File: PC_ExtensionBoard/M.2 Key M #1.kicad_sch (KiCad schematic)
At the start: 14 parts, among them J5 Bus_M.2_MDT180M03001

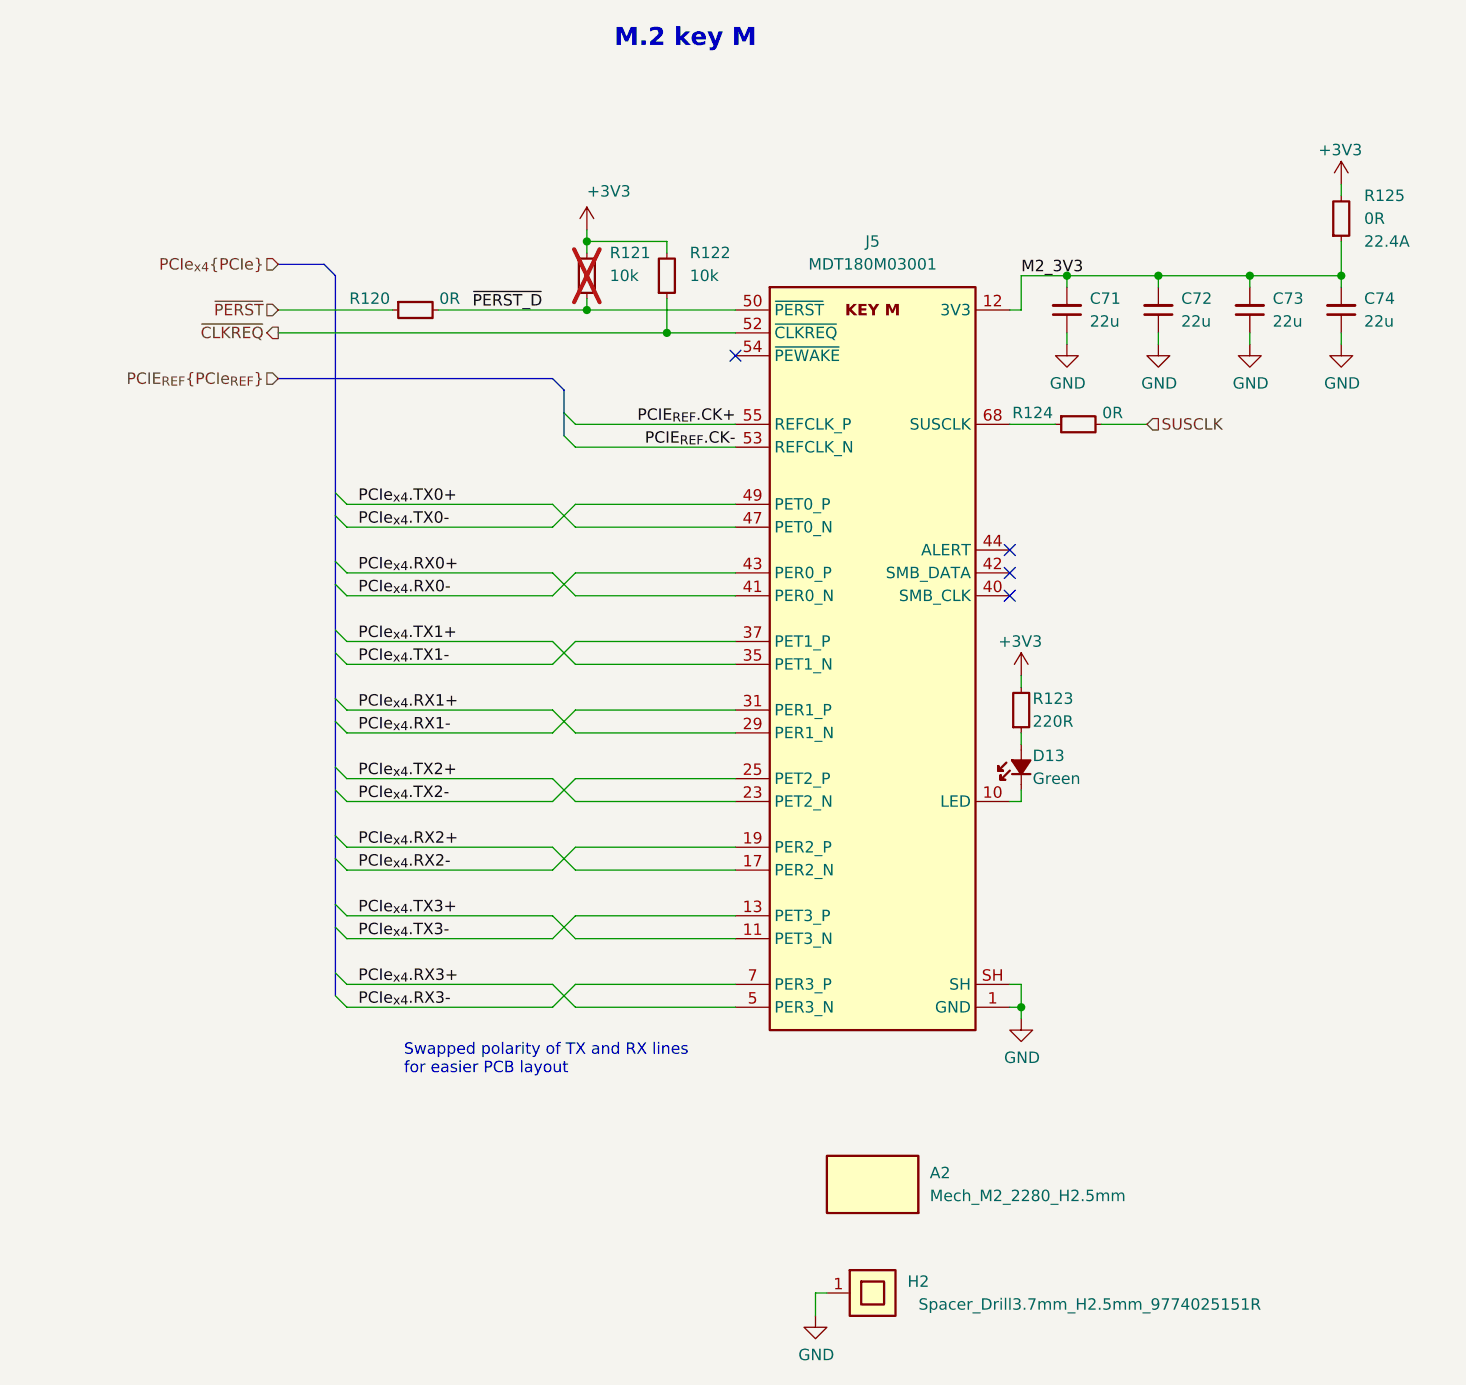
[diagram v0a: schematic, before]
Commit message: components placement R1
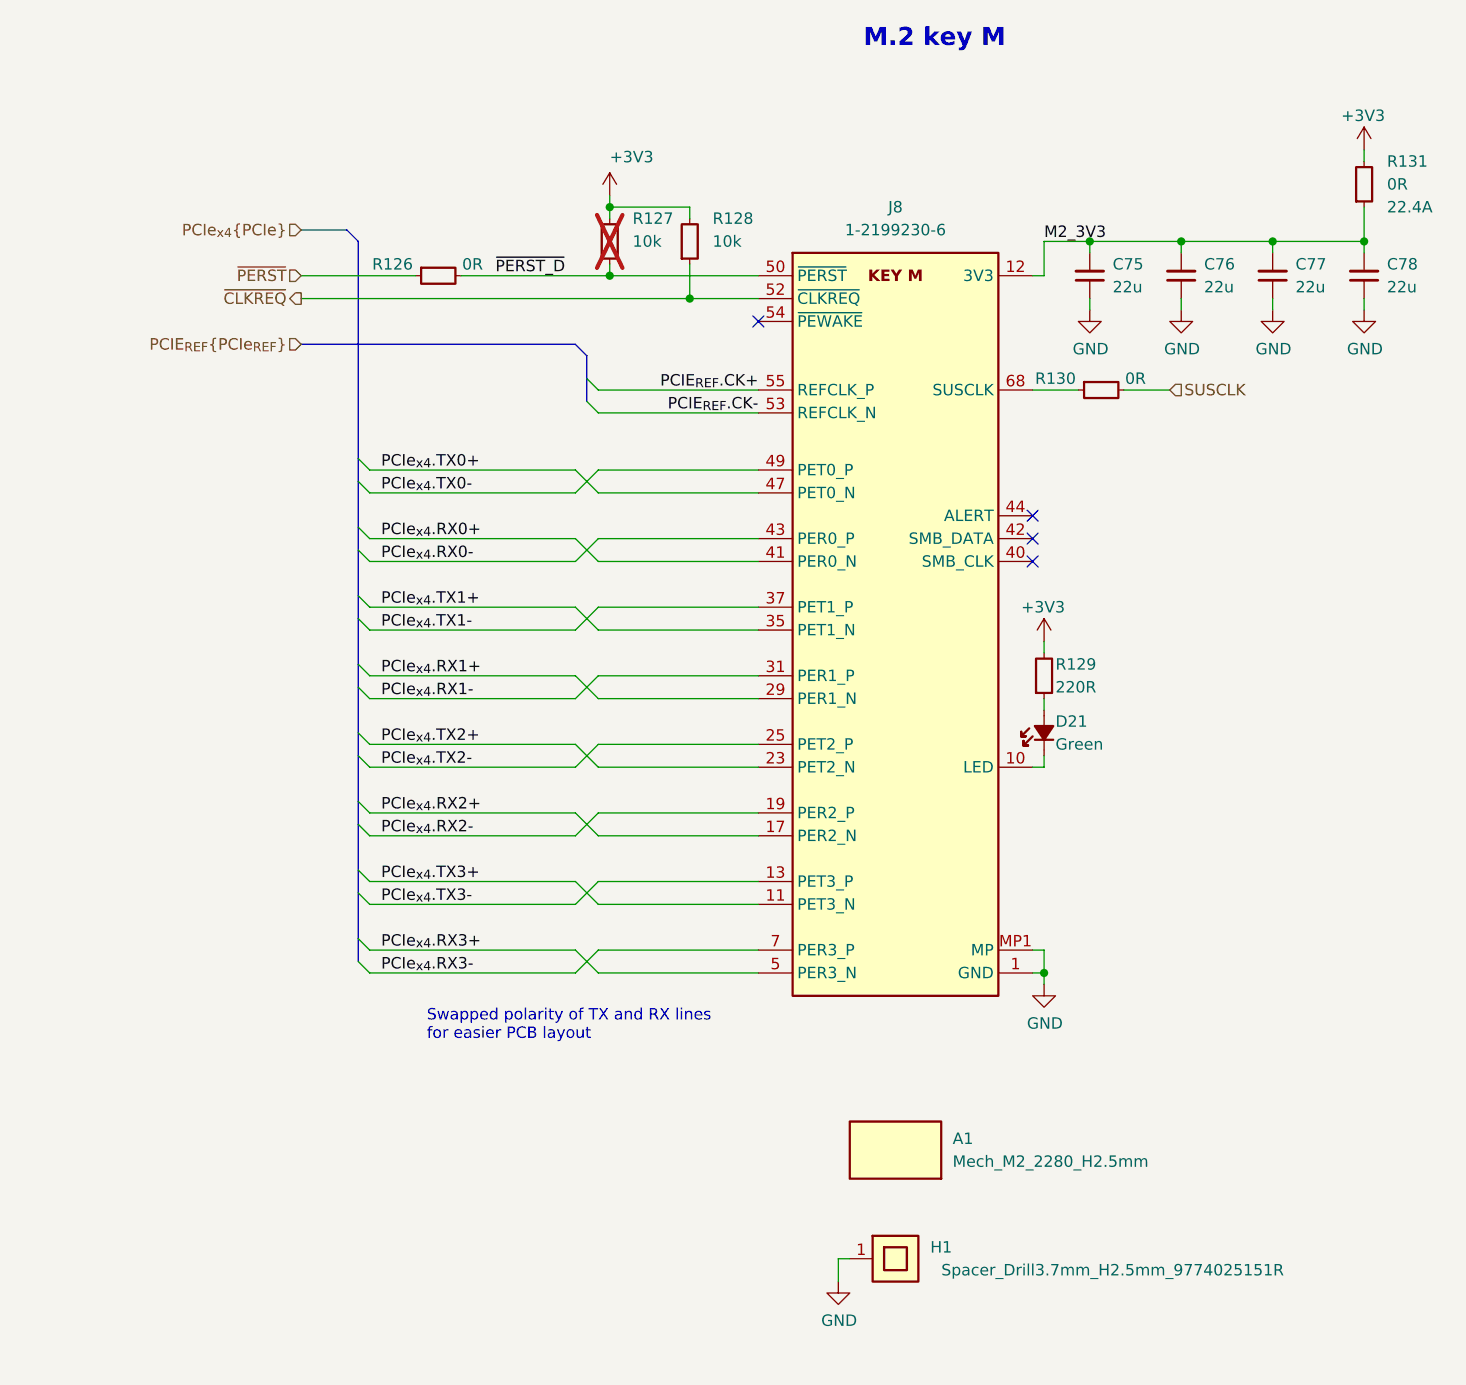
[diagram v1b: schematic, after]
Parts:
- removed A2: Mech_M2_2280_H2.5mm, antmicro-footprints:Mech_M2_2280_H2.5mm, symbol antmicroModules:Mech_M2_2280_H2.5mm
- removed C71, C72, C73, C74: C_22u_16V_0603, antmicro-footprints:C_0603_1608Metric, symbol antmicroCapacitors0603:C_22u_16V_0603
- removed D13: LED_G_0603_LTST-C190GKT, antmicro-footprints:LED_0603_1608Metric_G, symbol antmicroLEDIndicationDiscrete:LED_G_0603_LTST-C190GKT
- removed H2: Spacer_Drill3.7mm_H2.5mm_9774025151R, antmicro-footprints:Spacer_Drill3.7mm_H2.5mm_9774025151R, symbol antmicroMechanicalParts:Spacer_Drill3.7mm_H2.5mm_9774025151R
- removed J5: Bus_M.2_MDT180M03001, antmicro-footprints:Bus_M.2_Socket_Key_M_Amphenol_MDT180M03001, symbol antmicroPciConnectors:Bus_M.2_MDT180M03001
- removed R120, R124: R_0R_0402, antmicro-footprints:R_0402_1005Metric, symbol antmicroResistors0402:R_0R_0402
- removed R121, R122: R_10k_0402, antmicro-footprints:R_0402_1005Metric, symbol antmicroResistors0402:R_10k_0402
- removed R123: R_220R_0402, antmicro-footprints:R_0402_1005Metric, symbol antmicroResistors0402:R_220R_0402
- removed R125: R_0R_22.4A_0603, antmicro-footprints:R_0603_1608Metric, symbol antmicroResistors0603:R_0R_22.4A_0603
- added A1: Mech_M2_2280_H2.5mm, PC_Components_1:Mech_M2_2280_H2.5mm, symbol antmicroModules:Mech_M2_2280_H2.5mm
- added C75, C76, C77, C78: C_22u_16V_0603, PC_Components_1:C_0603_1608Metric, symbol antmicroCapacitors0603:C_22u_16V_0603
- added D21: LED_G_0603_LTST-C190GKT, PC_Components_1:LED_0603_1608Metric_G, symbol antmicroLEDIndicationDiscrete:LED_G_0603_LTST-C190GKT
- added H1: Spacer_Drill3.7mm_H2.5mm_9774025151R, PC_Components_1:Spacer_Drill3.7mm_H2.5mm_9774025151R, symbol antmicroMechanicalParts:Spacer_Drill3.7mm_H2.5mm_9774025151R
- added J8: Bus_M.2_1-2199230-6, PC_Components_1:Bus_M.2_Socket_Key_M_TE_1-2199230-6, symbol antmicroPciConnectors:Bus_M.2_1-2199230-6
- added R126, R130: R_0R_0402, PC_Components_1:R_0402_1005Metric, symbol antmicroResistors0402:R_0R_0402
- added R127, R128: R_10k_0402, PC_Components_1:R_0402_1005Metric, symbol antmicroResistors0402:R_10k_0402
- added R129: R_220R_0402, PC_Components_1:R_0402_1005Metric, symbol antmicroResistors0402:R_220R_0402
- added R131: R_0R_22.4A_0603, PC_Components_1:R_0603_1608Metric, symbol antmicroResistors0603:R_0R_22.4A_0603
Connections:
- net +3V3: now also R127.2, R128.2, R129.2, R131.2
- net GND: now also C75.1, C76.1, C77.1, C78.1, H1.1, J8.1 (GND), J8.15 (GND), J8.21 (GND), J8.27 (GND), J8.3 (GND), J8.33 (GND), J8.39 (GND), J8.45 (GND), J8.51 (GND), J8.57 (GND), J8.71 (GND), J8.73 (GND), J8.75 (GND), J8.9 (GND), J8.MP1 (MP), J8.MP2 (MP)
- net M2_3V3: now also C75.2, C76.2, C77.2, C78.2, J8.12 (3V3), J8.14 (3V3), J8.16 (3V3), J8.18 (3V3), J8.2 (3V3), J8.4 (3V3), J8.70 (3V3), J8.72 (3V3), J8.74 (3V3), R131.1
- net PCIE_{REF}.CK+: now also J8.55 (REFCLK_P)
- net PCIE_{REF}.CK-: now also J8.53 (REFCLK_N)
- net PCIe_{x4}.RX0+: now also J8.41 (PER0_N)
- net PCIe_{x4}.RX0-: now also J8.43 (PER0_P)
- net PCIe_{x4}.RX1+: now also J8.29 (PER1_N)
- net PCIe_{x4}.RX1-: now also J8.31 (PER1_P)
- net PCIe_{x4}.RX2+: now also J8.17 (PER2_N)
- net PCIe_{x4}.RX2-: now also J8.19 (PER2_P)
- net PCIe_{x4}.RX3+: now also J8.5 (PER3_N)
- net PCIe_{x4}.RX3-: now also J8.7 (PER3_P)
- net PCIe_{x4}.TX0+: now also J8.47 (PET0_N)
- net PCIe_{x4}.TX0-: now also J8.49 (PET0_P)
- net PCIe_{x4}.TX1+: now also J8.35 (PET1_N)
- net PCIe_{x4}.TX1-: now also J8.37 (PET1_P)
- net PCIe_{x4}.TX2+: now also J8.23 (PET2_N)
- net PCIe_{x4}.TX2-: now also J8.25 (PET2_P)
- net PCIe_{x4}.TX3+: now also J8.11 (PET3_N)
- net PCIe_{x4}.TX3-: now also J8.13 (PET3_P)
- net SUSCLK: now also R130.2
- net ~{CLKREQ}: now also J8.52 (~{CLKREQ}), R128.1
- net ~{PERST_D}: now also J8.50 (~{PERST}), R126.2, R127.1
- net ~{PERST}: now also R126.1
- new net: D21.2 (A), R129.1
- new net: J8.68 (SUSCLK), R130.1
- new net: D21.1 (C), J8.10 (LED)
